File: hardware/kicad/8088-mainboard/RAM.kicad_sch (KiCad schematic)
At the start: 4 parts, among them U13 HM62256BLP, U9 HM62256BLP

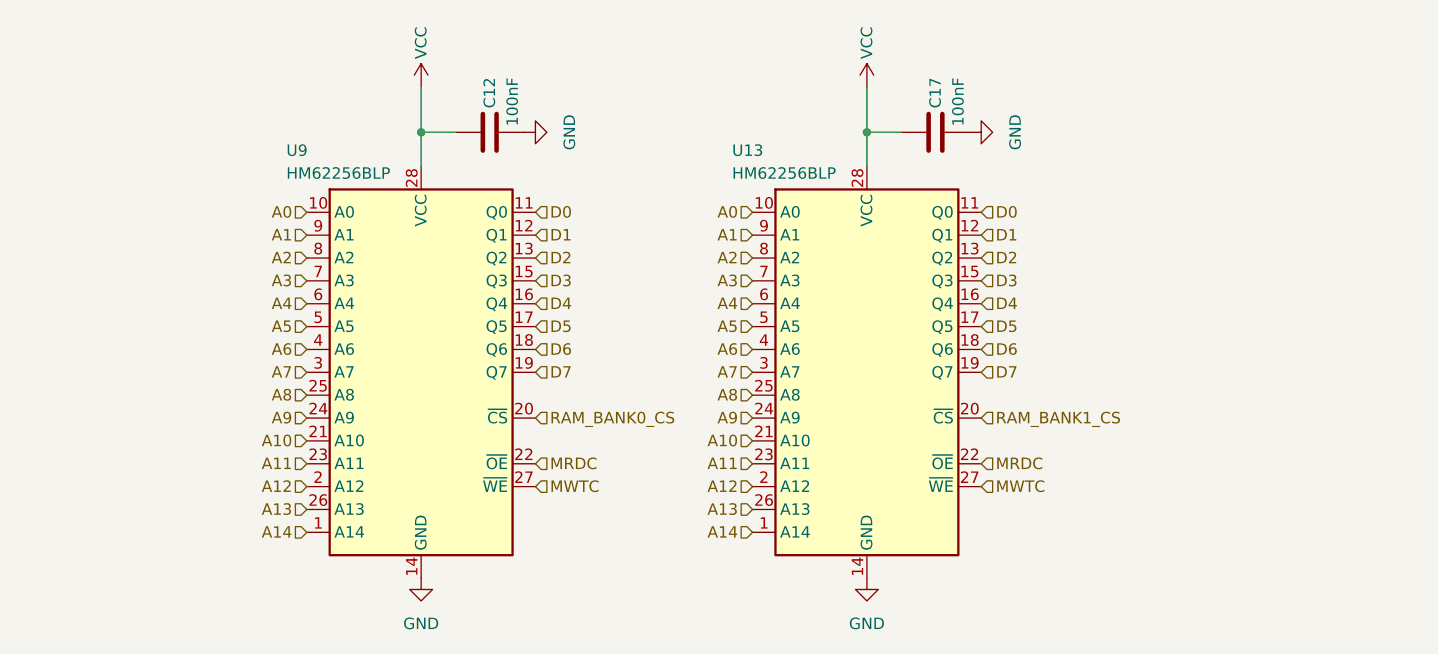
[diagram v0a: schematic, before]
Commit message: Update 8086-mainboard scheme
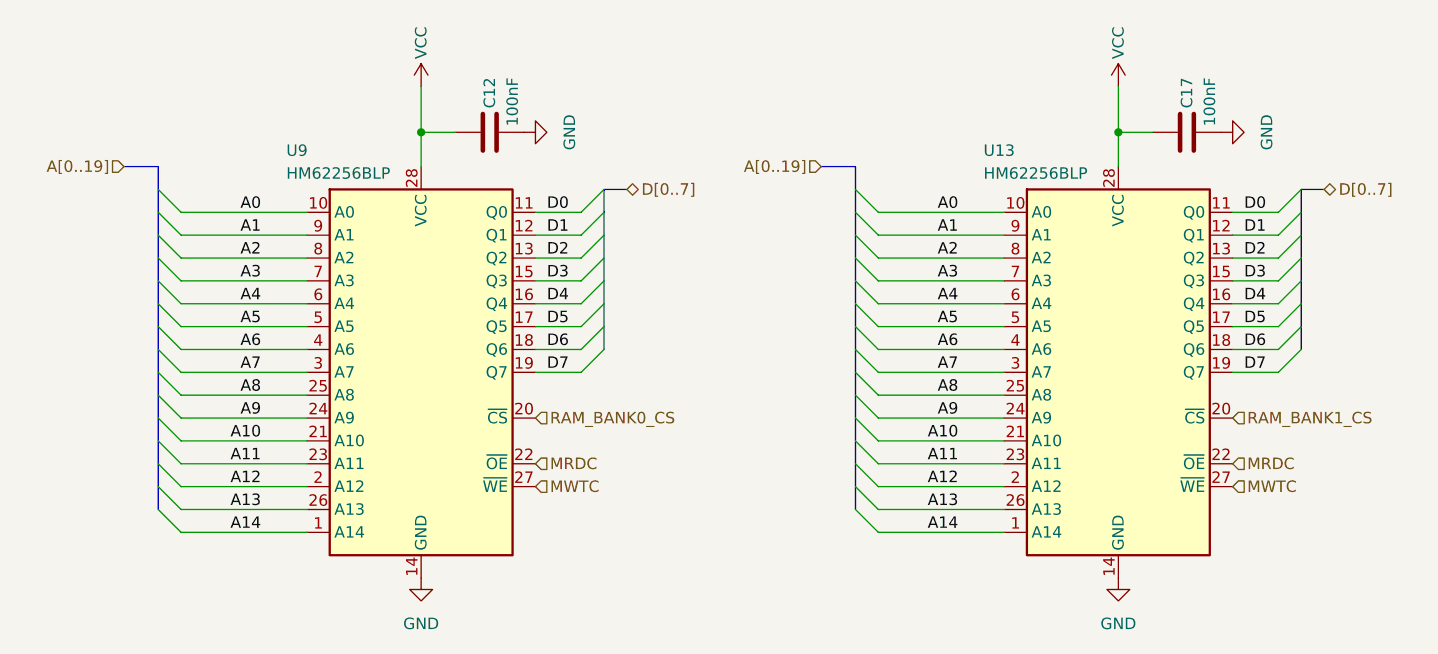
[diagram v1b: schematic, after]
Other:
- moved on the sheet: C17, U13
